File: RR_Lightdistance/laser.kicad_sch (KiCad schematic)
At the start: 1 part

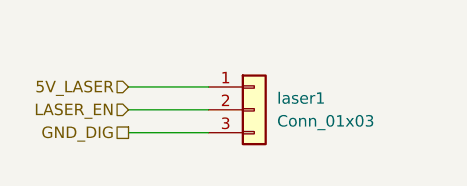
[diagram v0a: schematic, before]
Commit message: starting pcb
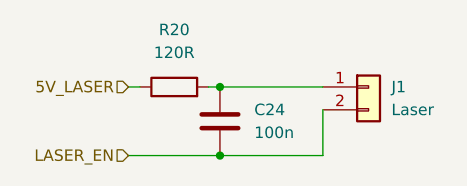
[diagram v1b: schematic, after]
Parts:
- removed laser1: Conn_01x03, symbol Connector_Generic:Conn_01x03
- added C24: 100n, Capacitor_SMD:C_0603_1608Metric, symbol Device:C
- added J1: Laser, Connector_JST:JST_PH_B2B-PH-K_1x02_P2.00mm_Vertical, symbol Connector_Generic:Conn_01x02
- added R20: 120R, Resistor_SMD:R_0805_2012Metric, symbol Device:R
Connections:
- net 5V_LASER: now also R20.1
- net LASER_EN: now also C24.2, J1.2 (Pin_2)
- new net: C24.1, J1.1 (Pin_1), R20.2
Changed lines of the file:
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@@
 	(generator_version "10.0")
 	(paper "A4")
-	(wire
-		(pts
-			(xy 138.43 86.36) (xy 147.32 86.36)
-		)
-		(stroke
-			(width 0)
-			(type default)
-		)
-	)
-	(wire
-		(pts
-			(xy 147.32 88.9) (xy 138.43 88.9)
-		)
-		(stroke
-			(width 0)
-			(type default)
-		)
-	)
-	(wire
-		(pts
-			(xy 147.32 83.82) (xy 138.43 83.82)
+	(junction
+		(at 148.59 91.44)
+		(diameter 0)
+		(color 0 0 0 0)
+	)
+	(junction
+		(at 148.59 83.82)
+		(diameter 0)
+		(color 0 0 0 0)
+	)
+	(wire
+		(pts
+			(xy 138.43 91.44) (xy 148.59 91.44)
+		)
+		(stroke
+			(width 0)
+			(type default)
+		)
+	)
+	(wire
+		(pts
+			(xy 147.32 83.82) (xy 148.59 83.82)
+		)
+		(stroke
+			(width 0)
+			(type default)
+		)
+	)
+	(wire
+		(pts
+			(xy 148.59 83.82) (xy 160.02 83.82)
+		)
+		(stroke
+			(width 0)
+			(type default)
+		)
+	)
+	(wire
+		(pts
+			(xy 160.02 91.44) (xy 148.59 91.44)
+		)
+		(stroke
+			(width 0)
+			(type default)
+		)
+	)
+	(wire
+		(pts
+			(xy 160.02 86.36) (xy 160.02 91.44)
+		)
+		(stroke
+			(width 0)
+			(type default)
+		)
+	)
+	(wire
+		(pts
+			(xy 138.43 83.82) (xy 139.7 83.82)
 		)
 		(stroke
@@
 	(hierarchical_label "LASER_EN"
 		(shape input)
-		(at 138.43 86.36 180)
-		(effects
-			(font
-				(size 1.27 1.27)
-			)
-			(justify right)
-		)
-	)
-	(hierarchical_label "GND_DIG"
-		(shape passive)
-		(at 138.43 88.9 180)
+		(at 138.43 91.44 180)
 		(effects
 			(font
@@
 	)
 	(symbol
-		(lib_id "Connector_Generic:Conn_01x03")
-		(at 152.4 86.36 0)
+		(lib_id "Connector_Generic:Conn_01x02")
+		(at 165.1 83.82 0)
 		(unit 1)
 		(body_style 1)
@@
 		(dnp no)
 		(fields_autoplaced yes)
-		(property "Reference" "laser1"
-			(at 154.94 85.0899 0)
+		(property "Reference" "J1"
+			(at 167.64 83.8199 0)
 			(show_name no)
 			(do_not_autoplace no)
@@
 			)
 		)
-		(property "Value" "Conn_01x03"
-			(at 154.94 87.6299 0)
+		(property "Value" "Laser"
+			(at 167.64 86.3599 0)
 			(show_name no)
 			(do_not_autoplace no)
@@
 			)
 		)
-		(property "Footprint" ""
-			(at 152.4 86.36 0)
+		(property "Footprint" "Connector_JST:JST_PH_B2B-PH-K_1x02_P2.00mm_Vertical"
+			(at 165.1 83.82 0)
 			(hide yes)
 			(show_name no)
@@
 		)
 		(property "Datasheet" ""
-			(at 152.4 86.36 0)
-			(hide yes)
-			(show_name no)
-			(do_not_autoplace no)
-			(effects
-				(font
-					(size 1.27 1.27)
-				)
-			)
-		)
-		(property "Description" "Generic connector, single row, 01x03, script generated (kicad-library-utils/schlib/autogen/connector/)"
-			(at 152.4 86.36 0)
-			(hide yes)
-			(show_name no)
-			(do_not_autoplace no)
-			(effects
-				(font
-					(size 1.27 1.27)
-				)
-			)
-		)
-		(pin "3"
+			(at 165.1 83.82 0)
+			(hide yes)
+			(show_name no)
+			(do_not_autoplace no)
+			(effects
+				(font
+					(size 1.27 1.27)
+				)
+			)
+		)
+		(property "Description" "Generic connector, single row, 01x02, script generated (kicad-library-utils/schlib/autogen/connector/)"
+			(at 165.1 83.82 0)
+			(hide yes)
+			(show_name no)
+			(do_not_autoplace no)
+			(effects
+				(font
+					(size 1.27 1.27)
+				)
+			)
 		)
 		(pin "1"
@@
 			(project "RR_Lightdistance"
 				(path "/29467ab3-c1bf-4fb3-96d7-e47c1d2d2674/e236e126-592c-40f1-8fdc-6421fbbe8784"
-					(reference "laser1")
+					(reference "J1")
 					(unit 1)
 				)
+			)
+		)
+	)
+	(symbol
+		(lib_id "Device:C")
+		(at 148.59 87.63 0)
+		(unit 1)
+		(body_style 1)
+		(exclude_from_sim no)
+		(in_bom yes)
+		(on_board yes)
+		(in_pos_files yes)
+		(dnp no)
+		(fields_autoplaced yes)
+		(property "Reference" "C24"
+			(at 152.4 86.3599 0)
+			(show_name no)
+			(do_not_autoplace no)
+			(effects
+				(font
+					(size 1.27 1.27)
+				)
+				(justify left)
+			)
+		)
+		(property "Value" "100n"
+			(at 152.4 88.8999 0)
+			(show_name no)
+			(do_not_autoplace no)
+			(effects
+				(font
+					(size 1.27 1.27)
+				)
+				(justify left)
+			)
+		)
+		(property "Footprint" "Capacitor_SMD:C_0603_1608Metric"
+			(at 149.5552 91.44 0)
+			(hide yes)
+			(show_name no)
+			(do_not_autoplace no)
+			(effects
+				(font
+					(size 1.27 1.27)
+				)
+			)
+		)
+		(property "Datasheet" ""
+			(at 148.59 87.63 0)
+			(hide yes)
+			(show_name no)
+			(do_not_autoplace no)
+			(effects
+				(font
+					(size 1.27 1.27)
+				)
+			)
+		)
+		(property "Description" "Unpolarized capacitor"
+			(at 148.59 87.63 0)
+			(hide yes)
+			(show_name no)
+			(do_not_autoplace no)
+			(effects
+				(font
+					(size 1.27 1.27)
+				)
+			)
+		)
+		(pin "2"
+		)
+		(pin "1"
+		)
+		(instances
+			(project "RR_Lightdistance"
+				(path "/29467ab3-c1bf-4fb3-96d7-e47c1d2d2674/e236e126-592c-40f1-8fdc-6421fbbe8784"
+					(reference "C24")
+					(unit 1)
+				)
+			)
+		)
+	)
+	(symbol
+		(lib_id "Device:R")
+		(at 143.51 83.82 90)
+		(unit 1)
+		(body_style 1)
+		(exclude_from_sim no)
+		(in_bom yes)
+		(on_board yes)
+		(in_pos_files yes)
+		(dnp no)
+		(fields_autoplaced yes)
+		(property "Reference" "R20"
+			(at 143.51 77.47 90)
+			(show_name no)
+			(do_not_autoplace no)
+			(effects
+				(font
+					(size 1.27 1.27)
+				)
+			)
+		)
+		(property "Value" "120R"
+			(at 143.51 80.01 90)
+			(show_name no)
+			(do_not_autoplace no)
+			(effects
+				(font
+					(size 1.27 1.27)
+				)
+			)
+		)
+		(property "Footprint" "Resistor_SMD:R_0805_2012Metric"
+			(at 143.51 85.598 90)
+			(hide yes)
+			(show_name no)
+			(do_not_autoplace no)
+			(effects
+				(font
+					(size 1.27 1.27)
+				)
+			)
+		)
+		(property "Datasheet" ""
+			(at 143.51 83.82 0)
+			(hide yes)
+			(show_name no)
+			(do_not_autoplace no)
+			(effects
+				(font
+					(size 1.27 1.27)
+				)
+			)
+		)
+		(property "Description" "Resistor"
+			(at 143.51 83.82 0)
+			(hide yes)
+			(show_name no)
+			(do_not_autoplace no)
+			(effects
+				(font
+					(size 1.27 1.27)
+				)
+			)
+		)
+		(pin "2"
+		)
+		(pin "1"
+		)
+		(instances
+			(project "RR_Lightdistance"
+				(path "/29467ab3-c1bf-4fb3-96d7-e47c1d2d2674/e236e126-592c-40f1-8fdc-6421fbbe8784"
+					(reference "R20")
+					(unit 1)
+				)
